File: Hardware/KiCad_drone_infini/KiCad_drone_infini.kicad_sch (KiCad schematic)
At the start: 21 parts, among them IC1 TESEO-LIV3R, IC3 L4973D5.1-013TR, J1 Conn_01x03, J2 Conn_01x03, J3 Conn_01x03, J4 Conn_01x03, U1 STM32H743VITx, U2 INA226, U3 LSM6DS3, U4 MPL3115A2

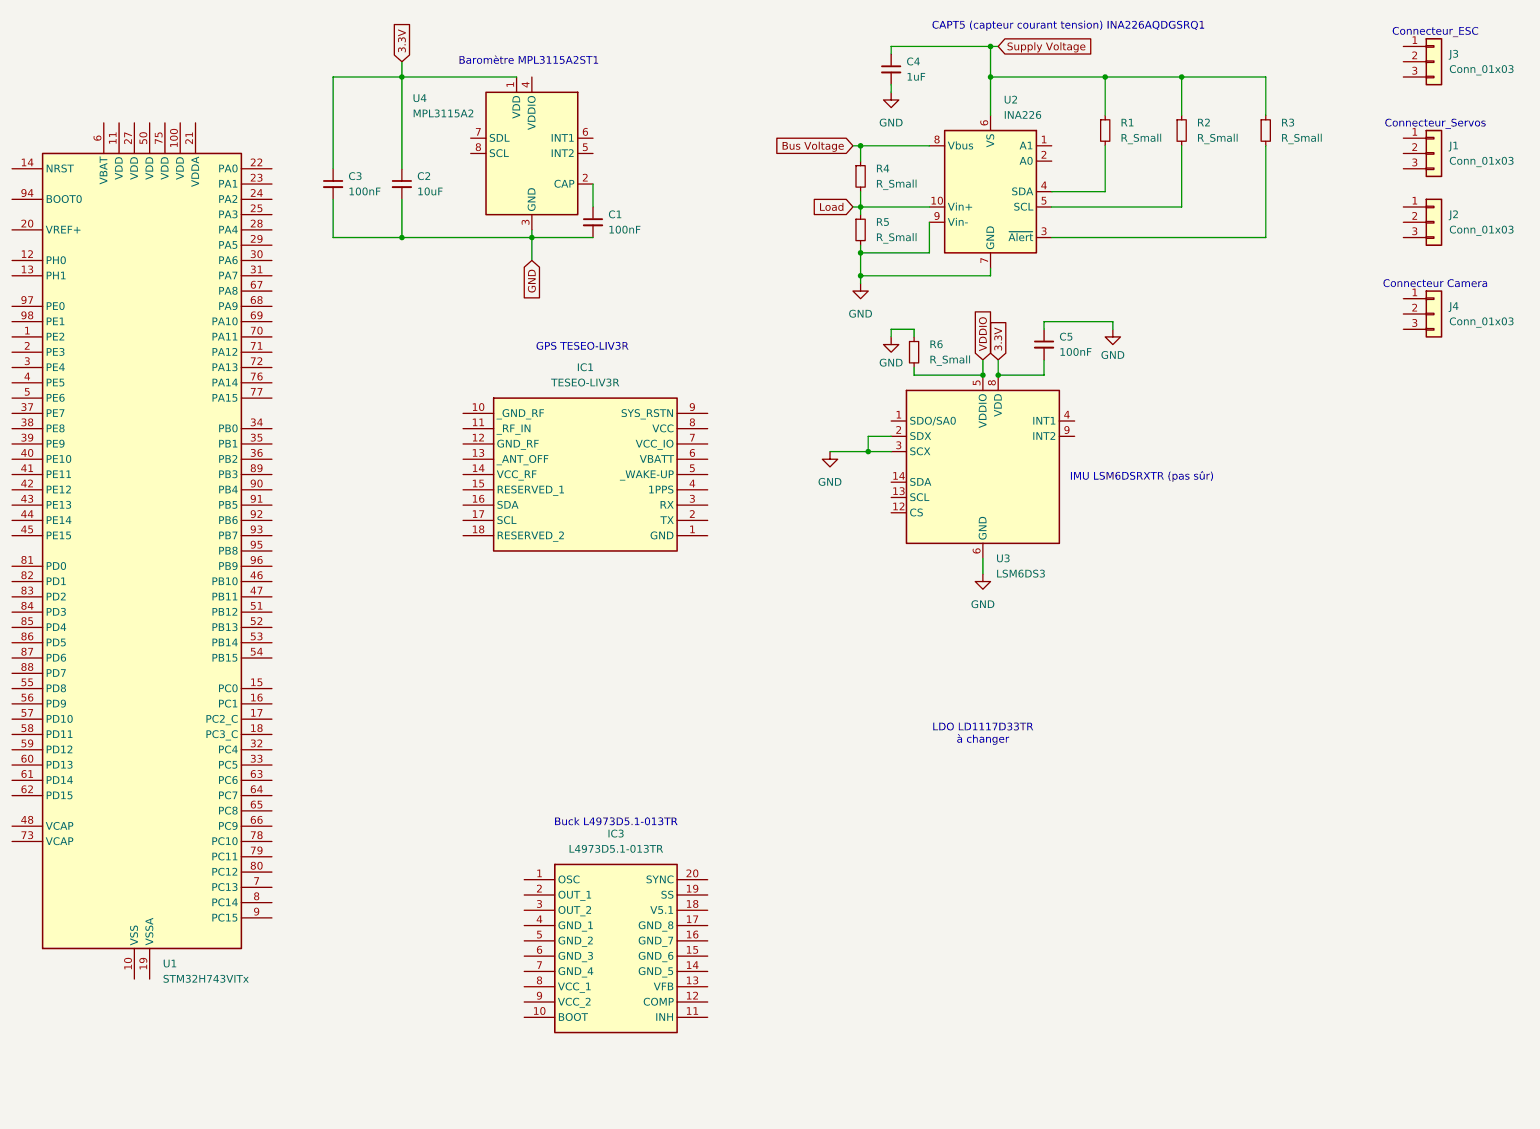
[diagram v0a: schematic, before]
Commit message: Modif Kicad 28/11
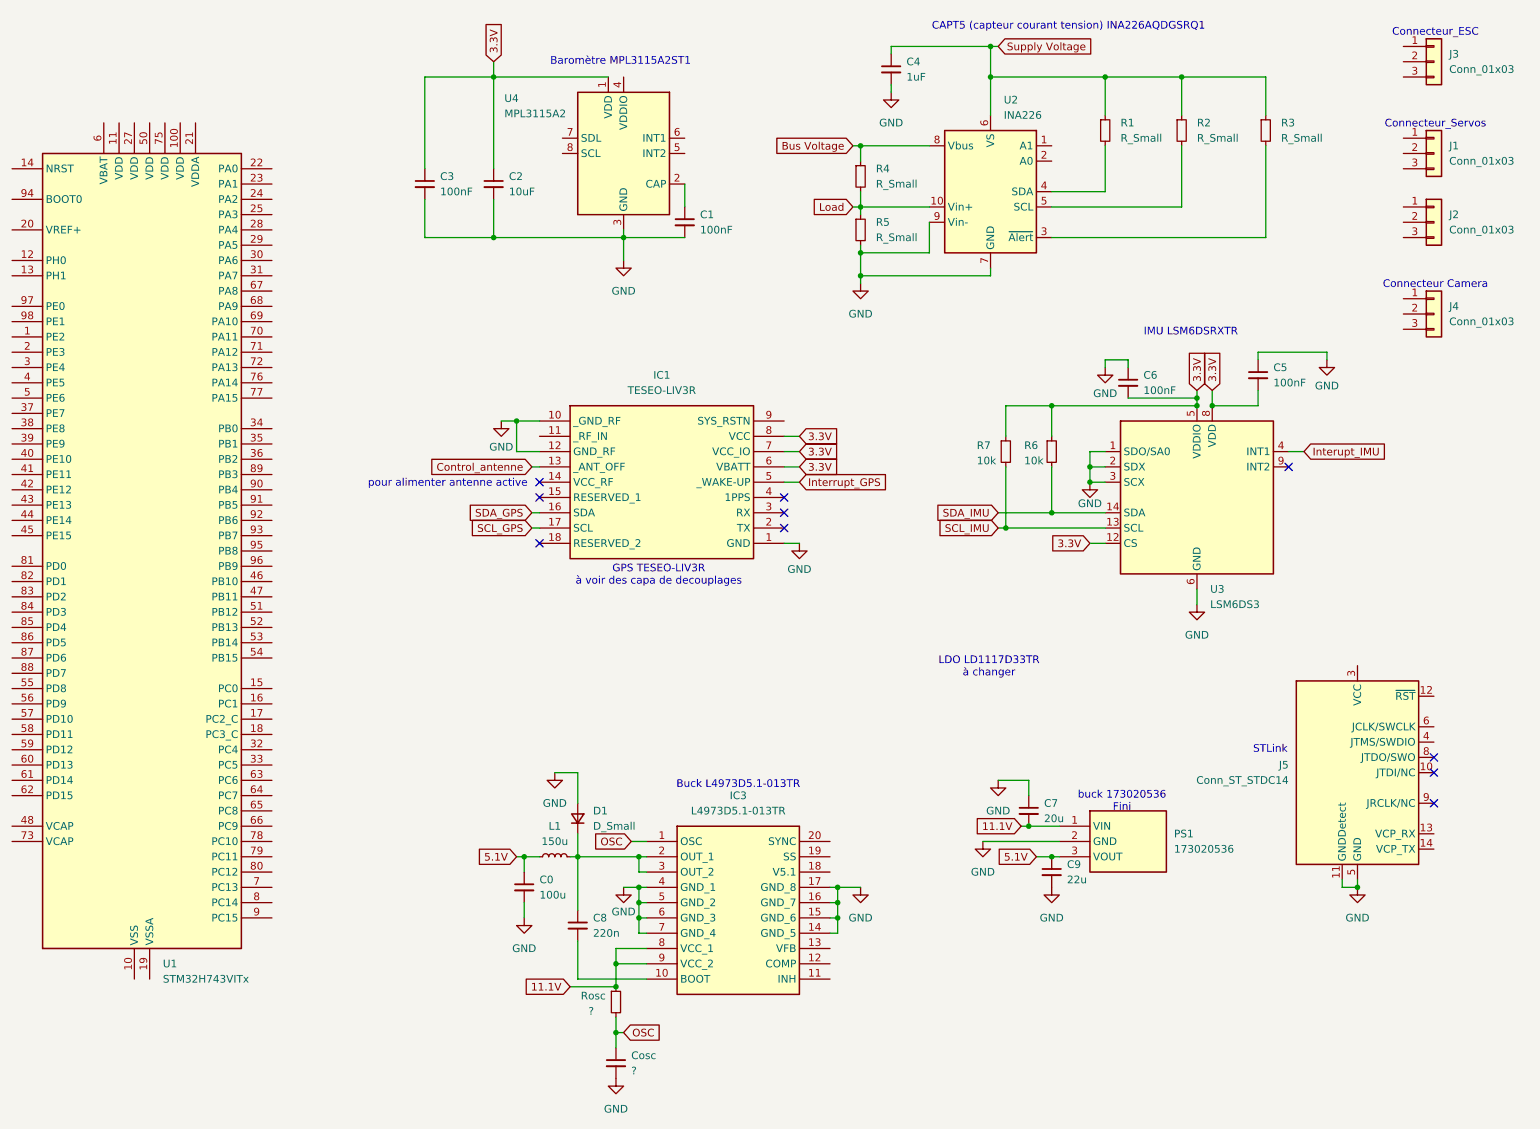
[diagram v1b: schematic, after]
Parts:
- added C0: 100u, symbol Device:C_Small
- added C6: 100nF, symbol Device:C_Small
- added C7: 20u, symbol Device:C_Small
- added C8: 220n, symbol Device:C_Small
- added C9: 22u, symbol Device:C_Small
- added Cosc: ?, symbol Device:C_Small
- added D1: D_Small, symbol Device:D_Small
- added J5: Conn_ST_STDC14, Connector_PinHeader_1.27mm:PinHeader_2x07_P1.27mm_Vertical_SMD, symbol Connector:Conn_ST_STDC14
- added L1: 150u, symbol Device:L_Small
- added PS1: 173020536, 173020536, symbol buck_173020536:173020536
- added R7: 10k, symbol Device:R_Small
- added Rosc: ?, symbol Device:R_Small
- R6: value R_Small -> 10k
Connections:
- net 3.3V: now also IC1.6 (VBATT), IC1.7 (VCC_IO), IC1.8 (VCC), R6.1, U3.12 (CS), U3.5 (VDDIO), C6.2, R7.1
- net GND: now also IC1.1 (GND), IC1.10 (_GND_RF), IC1.12 (GND_RF), IC3.14 (GND_5), IC3.15 (GND_6), IC3.16 (GND_7), IC3.17 (GND_8), IC3.4 (GND_1), IC3.5 (GND_2), IC3.6 (GND_3), IC3.7 (GND_4), U3.1 (SDO/SA0), C0.2, C6.1, C7.1, C9.2, Cosc.2, D1.2 (A), J5.11 (GNDDetect), J5.5 (GND), J5.7 (GND), PS1.2 (GND); no longer R6.1
- net SCL_IMU: now reaches U3.13 (SCL)
- net SCL_IMU: now also R7.2
- net SDA_IMU: now reaches U3.14 (SDA)
- net SDA_IMU: now also R6.2
- net Interupt_IMU: now reaches U3.4 (INT1)
- net Control_antenne: now reaches IC1.13 (_ANT_OFF)
- net SDA_GPS: now reaches IC1.16 (SDA)
- net SCL_GPS: now reaches IC1.17 (SCL)
- net Interrupt_GPS: now reaches IC1.5 (_WAKE-UP)
- net OSC: now reaches IC3.1 (OSC)
- net OSC: now also Cosc.1, Rosc.2
- net at IC3.10 (BOOT): now also C8.2
- net at IC3.2 (OUT_1): now also IC3.3 (OUT_2), C8.1, D1.1 (K), L1.2
- net 11.1V: now reaches IC3.8 (VCC_1)
- net 11.1V: now also IC3.9 (VCC_2), C7.2, PS1.1 (VIN), Rosc.1
- removed net VDDIO: R6.2, U3.5 (VDDIO)
- new net 5.1V: C0.1, C9.1, L1.1, PS1.3 (VOUT)
- no-connect marks 0 -> 10
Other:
- note added: "GPS TESEO-LIV3R à voir des capa de decouplages"
- note added: "IMU LSM6DSRXTR"
- note added: "STLink"
- note added: "buck 173020536 Fini"
- note added: "pour alimenter antenne active"
- note removed: "GPS TESEO-LIV3R"
- note removed: "IMU LSM6DSRXTR (pas sûr)"
- moved on the sheet: C1, C2, C3, C5, IC1, IC3, U3, U4
